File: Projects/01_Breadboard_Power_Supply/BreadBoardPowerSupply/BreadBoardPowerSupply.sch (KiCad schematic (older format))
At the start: 15 parts, among them J1 Barrel_Jack_Switch, J2 Conn_02x02_Odd_Even, J3 Conn_02x02_Odd_Even, SW1 SW_DPDT_x2, U1 LM7805_TO220

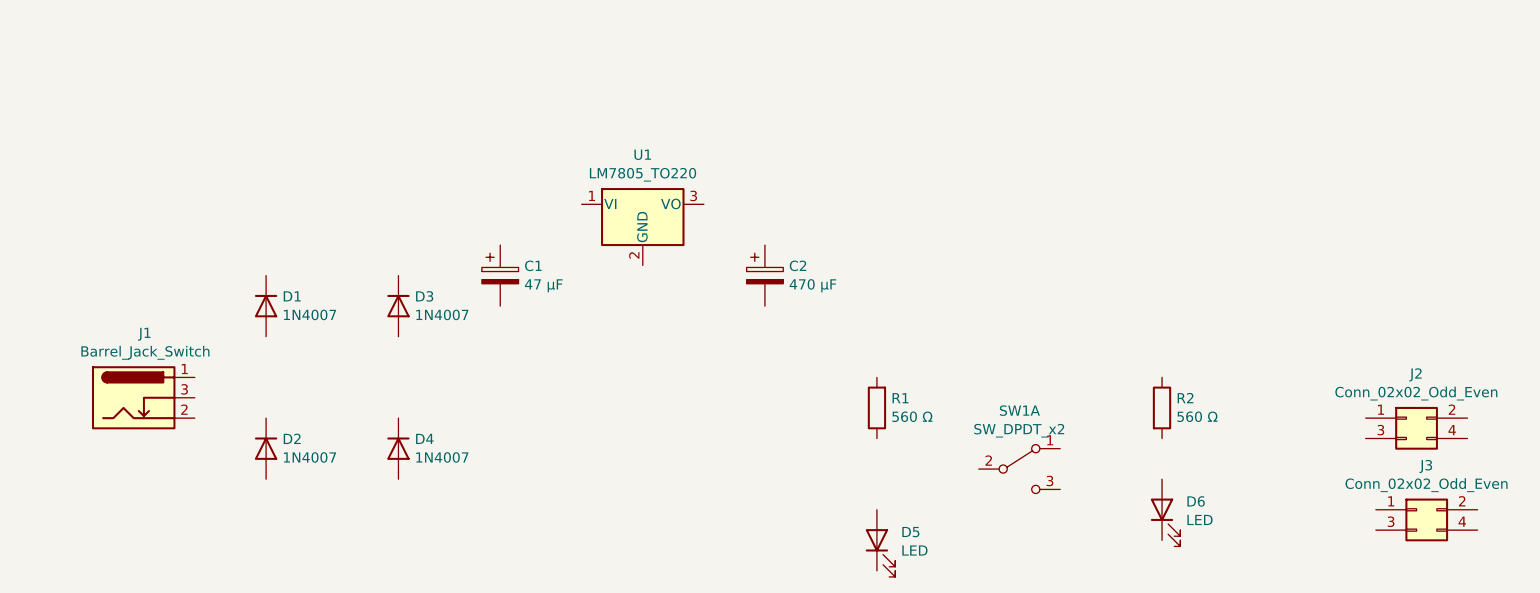
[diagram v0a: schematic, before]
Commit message: Wire Eeschema and run ERC
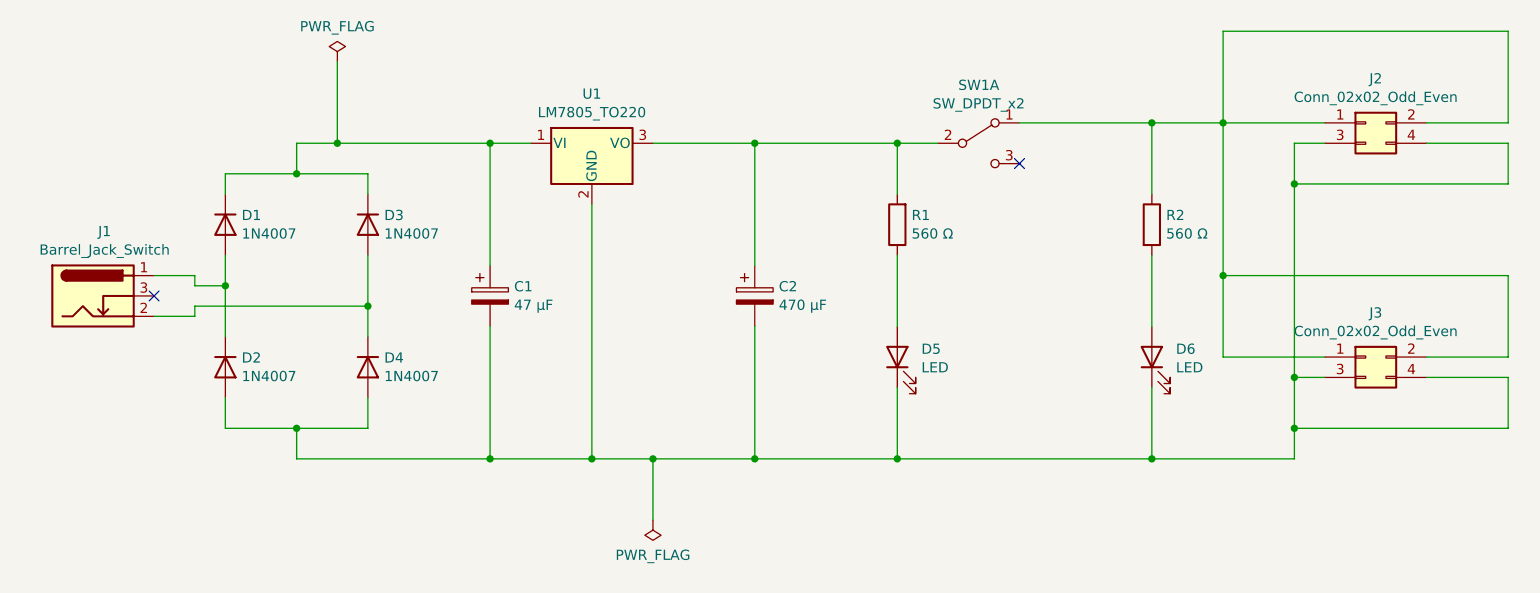
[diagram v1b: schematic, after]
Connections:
- net at C1.1: now also D1.1 (K), D3.1 (K), U1.1 (VI)
- net at C1.2: now also C2.2, D2.2 (A), D4.2 (A), D5.1 (K), D6.1 (K), J2.3 (Pin_3), J2.4 (Pin_4), J3.3 (Pin_3), J3.4 (Pin_4), U1.2 (GND)
- net at C2.1: now also R1.2, SW1.2 (B), U1.3 (VO)
- net at R2.1: now also J2.1 (Pin_1), J2.2 (Pin_2), J3.1 (Pin_1), J3.2 (Pin_2), SW1.1 (A)
- net at R2.2: now also D6.2 (A)
- net at D5.2 (A): now also R1.1
- net at D1.2 (A): now also D2.1 (K), J1.1
- net at D3.2 (A): now also D4.1 (K), J1.2
- no-connect marks 0 -> 2
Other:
- moved on the sheet: C1, C2, D1, D2, D3, D4, D5, D6, J1, J2, J3, R1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
